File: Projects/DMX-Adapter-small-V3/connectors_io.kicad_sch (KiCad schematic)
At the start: 11 parts, among them J1 USB_B_Micro, J2 USART, J3 SWD, J4 DMX, SW1 RST, SW2 BOOT0

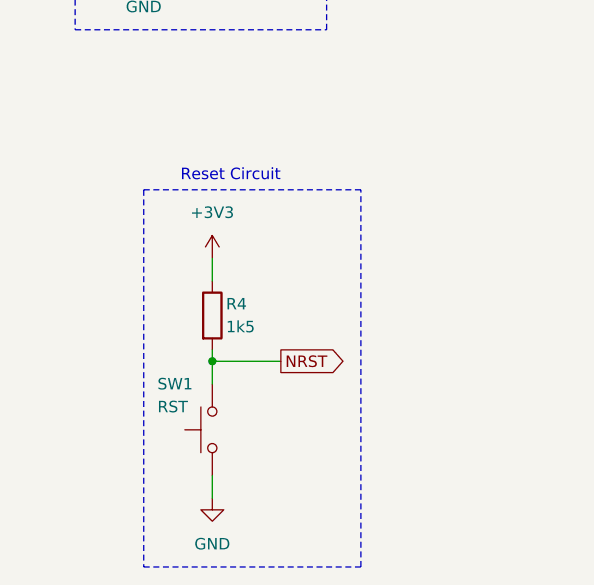
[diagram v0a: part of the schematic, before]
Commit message: final
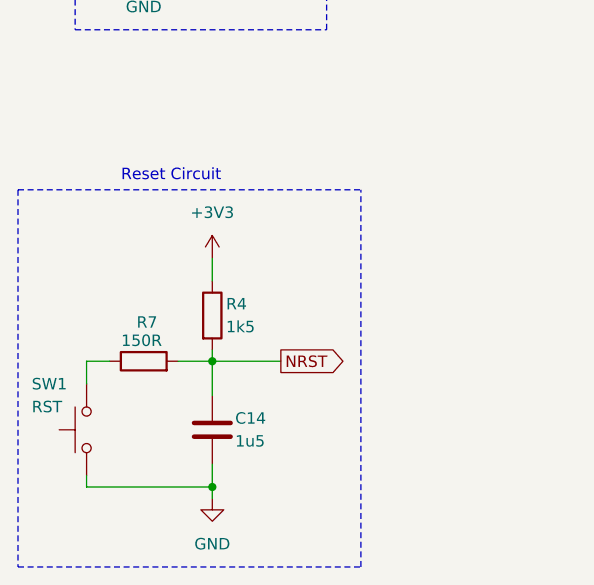
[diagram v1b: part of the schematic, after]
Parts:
- added C14: 1u5, Capacitor_SMD:C_0603_1608Metric, symbol Device:C
- added R7: 150R, Resistor_SMD:R_0402_1005Metric, symbol Device:R
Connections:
- net GND: now also C14.2
- net NRST: now also C14.1, R7.2; no longer SW1.2
- new net: R7.1, SW1.2
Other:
- moved on the sheet: SW1
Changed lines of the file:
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@@
 	(text "Reset Circuit"
 		(exclude_from_sim no)
-		(at 46.482 69.596 0)
+		(at 39.878 69.596 0)
 		(effects
 			(font
@@
 		(color 0 0 0 0)
 	)
+	(junction
+		(at 44.45 104.14)
+		(diameter 0)
+		(color 0 0 0 0)
+	)
 	(no_connect
 		(at 44.45 39.37)
@@
 		)
 	)
+	(wire
+		(pts
+			(xy 44.45 90.17) (xy 44.45 93.98)
+		)
+		(stroke
+			(width 0)
+			(type default)
+		)
+	)
 	(polyline
 		(pts
@@
 		)
 	)
+	(wire
+		(pts
+			(xy 30.48 102.87) (xy 30.48 104.14)
+		)
+		(stroke
+			(width 0)
+			(type default)
+		)
+	)
 	(polyline
 		(pts
@@
 	(polyline
 		(pts
-			(xy 36.83 113.03) (xy 60.96 113.03)
-		)
-		(stroke
-			(width 0)
-			(type dash)
+			(xy 22.86 113.03) (xy 60.96 113.03)
+		)
+		(stroke
+			(width 0)
+			(type dash)
+		)
+	)
+	(wire
+		(pts
+			(xy 30.48 90.17) (xy 30.48 92.71)
+		)
+		(stroke
+			(width 0)
+			(type default)
 		)
 	)
@@
 	(wire
 		(pts
+			(xy 40.64 90.17) (xy 44.45 90.17)
+		)
+		(stroke
+			(width 0)
+			(type default)
+		)
+	)
+	(wire
+		(pts
 			(xy 44.45 88.9) (xy 44.45 90.17)
 		)
@@
 	(wire
 		(pts
+			(xy 44.45 104.14) (xy 44.45 105.41)
+		)
+		(stroke
+			(width 0)
+			(type default)
+		)
+	)
+	(wire
+		(pts
 			(xy 132.08 34.29) (xy 132.08 33.02)
 		)
@@
 	(polyline
 		(pts
-			(xy 36.83 71.12) (xy 36.83 113.03)
+			(xy 22.86 71.12) (xy 22.86 113.03)
 		)
 		(stroke
@@
 	(wire
 		(pts
+			(xy 30.48 104.14) (xy 44.45 104.14)
+		)
+		(stroke
+			(width 0)
+			(type default)
+		)
+	)
+	(wire
+		(pts
 			(xy 92.71 69.85) (xy 92.71 72.39)
 		)
@@
 	(wire
 		(pts
-			(xy 44.45 102.87) (xy 44.45 105.41)
-		)
-		(stroke
-			(width 0)
-			(type default)
-		)
-	)
-	(wire
-		(pts
 			(xy 93.98 38.1) (xy 93.98 36.83)
 		)
@@
 	(polyline
 		(pts
-			(xy 36.83 71.12) (xy 60.96 71.12)
+			(xy 22.86 71.12) (xy 60.96 71.12)
 		)
 		(stroke
@@
 		)
 	)
+	(wire
+		(pts
+			(xy 33.02 90.17) (xy 30.48 90.17)
+		)
+		(stroke
+			(width 0)
+			(type default)
+		)
+	)
 	(polyline
 		(pts
@@
 	(wire
 		(pts
+			(xy 44.45 101.6) (xy 44.45 104.14)
+		)
+		(stroke
+			(width 0)
+			(type default)
+		)
+	)
+	(wire
+		(pts
 			(xy 149.86 38.1) (xy 149.86 35.56)
 		)
@@
 		(pts
 			(xy 167.64 76.2) (xy 167.64 74.93)
-		)
-		(stroke
-			(width 0)
-			(type default)
-		)
-	)
-	(wire
-		(pts
-			(xy 44.45 90.17) (xy 44.45 92.71)
 		)
 		(stroke
@@
 				(path "/ef5f791b-6275-4df9-ae9f-81fc9bb96b68/95f5c172-f812-45b1-82e4-e35a8bca5dd3"
 					(reference "#PWR05")
+					(unit 1)
+				)
+			)
+		)
+	)
+	(symbol
+		(lib_id "Device:C")
+		(at 44.45 97.79 0)
+		(unit 1)
+		(exclude_from_sim no)
+		(in_bom yes)
+		(on_board yes)
+		(dnp no)
+		(property "Reference" "C14"
+			(at 46.99 96.52 0)
+			(effects
+				(font
+					(size 1.27 1.27)
+				)
+				(justify left)
+			)
+		)
+		(property "Value" "1u5"
+			(at 46.99 99.06 0)
+			(effects
+				(font
+					(size 1.27 1.27)
+				)
+				(justify left)
+			)
+		)
+		(property "Footprint" "Capacitor_SMD:C_0603_1608Metric"
+			(at 45.4152 101.6 0)
+			(effects
+				(font
+					(size 1.27 1.27)
+				)
+				(hide yes)
+			)
+		)
+		(property "Datasheet" "https://www.mouser.de/ProductDetail/TDK/C1608X8L0J155K080AC?qs=sGAEpiMZZMuMW9TJLBQkXhEmpb63FTdUC9o8Bfzm4VU%3D"
+			(at 44.45 97.79 0)
+			(effects
+				(font
+					(size 1.27 1.27)
+				)
+				(hide yes)
+			)
+		)
+		(property "Description" "Unpolarized capacitor"
+			(at 44.45 97.79 0)
+			(effects
+				(font
+					(size 1.27 1.27)
+				)
+				(hide yes)
+			)
+		)
+		(property "Mouser-Nr" "810-C1608X8L0J155K08"
+			(at 44.45 97.79 0)
+			(effects
+				(font
+					(size 1.27 1.27)
+				)
+				(hide yes)
+			)
+		)
+		(pin "1"
+		)
+		(pin "2"
+		)
+		(instances
+			(project "DMX-Adapter-small-V3"
+				(path "/ef5f791b-6275-4df9-ae9f-81fc9bb96b68/95f5c172-f812-45b1-82e4-e35a8bca5dd3"
+					(reference "C14")
 					(unit 1)
 				)
@@
 	(symbol
 		(lib_id "Switch:SW_Push")
-		(at 44.45 97.79 90)
+		(at 30.48 97.79 90)
 		(unit 1)
 		(exclude_from_sim no)
@@
 		(dnp no)
 		(property "Reference" "SW1"
-			(at 38.354 92.71 90)
+			(at 24.384 92.71 90)
 			(effects
 				(font
@@
 		)
 		(property "Value" "RST"
-			(at 38.354 95.25 90)
+			(at 24.384 95.25 90)
 			(effects
 				(font
@@
 		)
 		(property "Footprint" "own:omron_B3U-1000P"
-			(at 39.37 97.79 0)
+			(at 25.4 97.79 0)
 			(effects
 				(font
@@
 		)
 		(property "Datasheet" "https://www.mouser.de/ProductDetail/Omron-Electronics/B3U-1000P?qs=AO7BQMcsEu4ip80xyf2FwA%3D%3D"
-			(at 39.37 97.79 0)
+			(at 25.4 97.79 0)
 			(effects
 				(font
@@
 		)
 		(property "Description" "Push button switch, generic, two pins"
-			(at 44.45 97.79 0)
+			(at 30.48 97.79 0)
 			(effects
 				(font
@@
 		)
 		(property "Mouser-Nr" "653-B3U-1000P"
-			(at 44.45 97.79 90)
+			(at 30.48 97.79 90)
 			(effects
 				(font
@@
 					(unit 1)
 				)
+			)
+		)
+	)
+	(symbol
+		(lib_id "Device:R")
+		(at 36.83 90.17 90)
+		(unit 1)
+		(exclude_from_sim no)
+		(in_bom yes)
+		(on_board yes)
+		(dnp no)
+		(property "Reference" "R7"
+			(at 38.354 85.852 90)
+			(effects
+				(font
+					(size 1.27 1.27)
+				)
+				(justify left)
+			)
+		)
+		(property "Value" "150R"
+			(at 38.862 87.884 90)
+			(effects
+				(font
+					(size 1.27 1.27)
+				)
+				(justify left)
+			)
+		)
+		(property "Footprint" "Resistor_SMD:R_0402_1005Metric"
+			(at 36.83 91.948 90)
+			(effects
+				(font
+					(size 1.27 1.27)
+				)
+				(hide yes)
+			)
+		)
+		(property "Datasheet" "https://www.mouser.de/ProductDetail/KOA-Speer/SG73P1EWTTP151J?qs=Jslch3jnSjnKow4tRGzcMQ%3D%3D"
+			(at 36.83 90.17 0)
+			(effects
+				(font
+					(size 1.27 1.27)
+				)
+				(hide yes)
+			)
+		)
+		(property "Description" "Resistor"
+			(at 36.83 90.17 0)
+			(effects
+				(font
+					(size 1.27 1.27)
+				)
+				(hide yes)
+			)
+		)
+		(property "Mouser-Nr" "660-SG73P1EWTTP151J"
+			(at 36.83 90.17 0)
+			(effects
+				(font
+					(size 1.27 1.27)
+				)
+				(hide yes)
+			)
+		)
+		(pin "2"
+		)
+		(pin "1"
+		)
+		(instances
+			(project "DMX-Adapter-small-V3"
+				(path "/ef5f791b-6275-4df9-ae9f-81fc9bb96b68/95f5c172-f812-45b1-82e4-e35a8bca5dd3"
+					(reference "R7")
+					(unit 1)
+				)
